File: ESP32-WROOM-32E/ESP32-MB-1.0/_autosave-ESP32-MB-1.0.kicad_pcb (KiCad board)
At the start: 2 copper layers, 125.6 x 91.4 mm, 52 parts, among them J1 Conn_01x19, J10 Conn_01x03_Pin, J11 Conn_01x03_Pin, J12 Conn_01x03_Pin, J13 Conn_01x03_Pin, J14 Conn_01x03_Pin, J15 Conn_01x03_Pin, J16 XT60-M, J2 Conn_01x19, J21 Conn_01x02_Pin, J22 XT60-M, J23 Conn_01x02_Pin, J24 Conn_01x02_Pin, J25 Conn_01x02_Pin, J26 Conn_01x02_Pin, J27 Conn_01x02_Pin, J28 Conn_01x02_Pin, J29 Conn_01x02_Pin, J3 Conn_01x19, J30 XT60-M, J31 Conn_01x02_Pin, J32 Conn_01x02_Pin, J33 Conn_01x11_Pin, J34 Conn_01x02_Pin, J35 Conn_01x02_Pin, J36 Conn_01x02_Pin, J37 Conn_01x02_Pin, J38 Conn_01x02_Pin, J39 Conn_01x02_Pin, J4 Conn_01x11_Pin, J5 Conn_01x11_Pin, J6 XT60-M, J7 Conn_01x19, J8 Conn_01x03_Pin, J9 Conn_01x03_Pin, U1 IRLB3813PBF, U2 IRLB3813PBF, U3 IRLB3813PBF, U4 IRLB3813PBF, U5 IRLB3813PBF, U6 IRLB3813PBF, U7 IRLB3813PBF, U8 IRLB3813PBF, U9 MCP2562-E-P

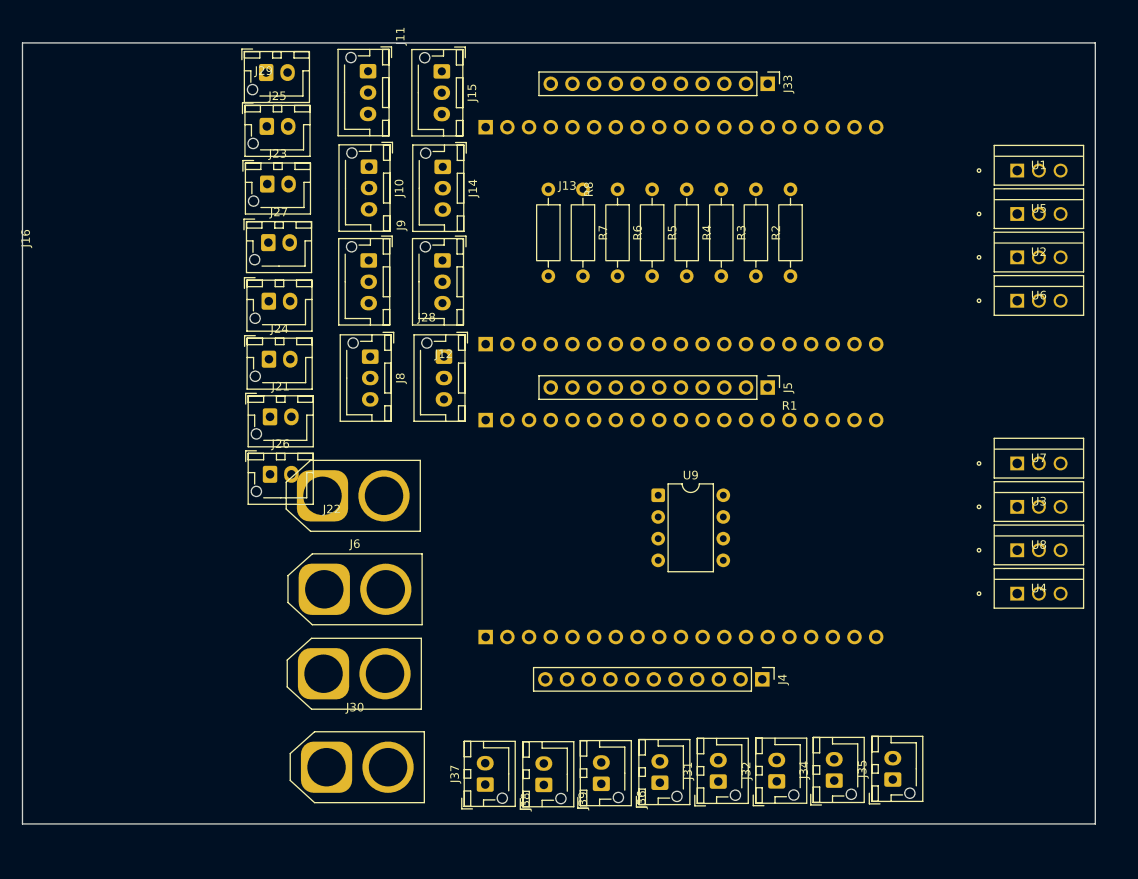
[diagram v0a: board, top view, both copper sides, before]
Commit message: ESP割り当て
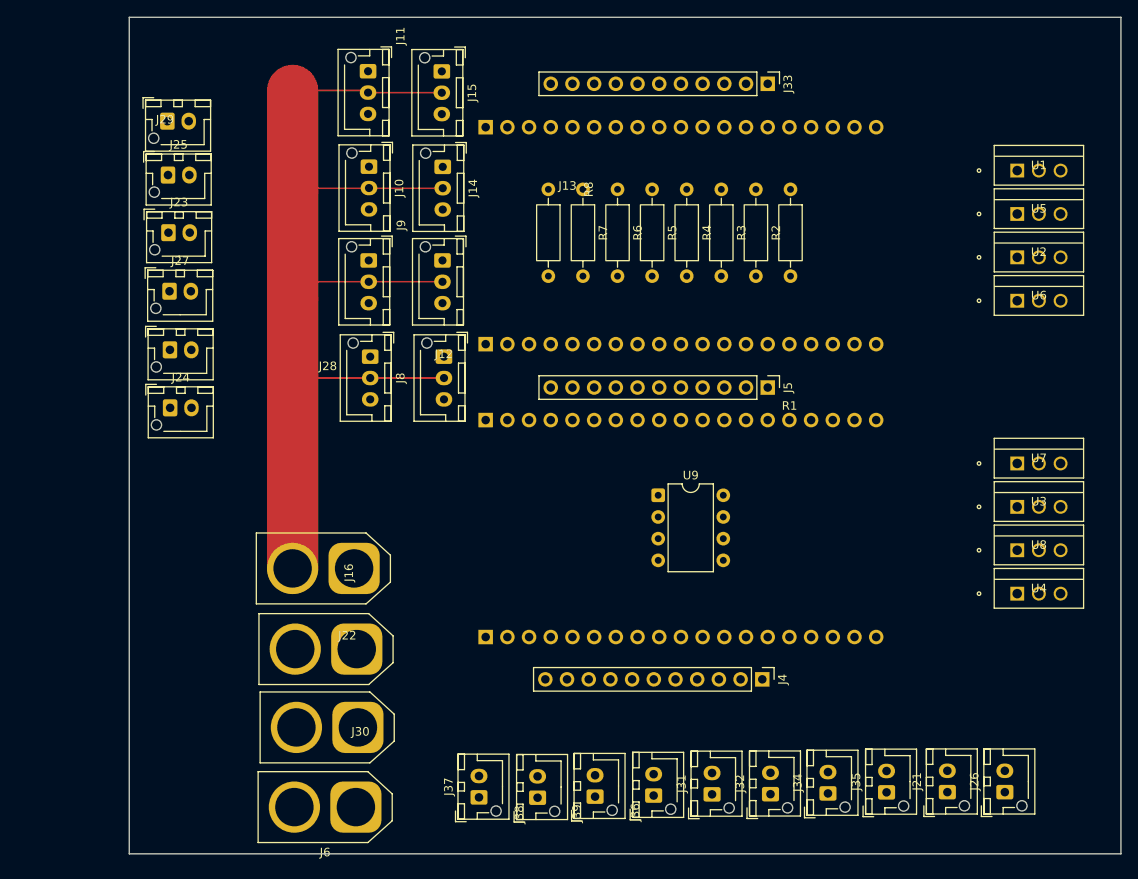
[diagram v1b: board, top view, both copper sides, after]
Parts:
- moved J26 93.7 mm to (234.0, 125.9), turned to 90 degrees
- moved J21 90.7 mm to (227.3, 125.9), turned to 90 degrees
- moved J6 25.8 mm to (158.0, 127.6), turned to 180 degrees
- moved J22 18.4 mm to (158.1, 109.1), turned to 180 degrees
- moved J28 12.9 mm to (136.3, 74.1)
- moved J23 12.9 mm to (136.1, 60.4)
- moved J25 12.9 mm to (136.0, 53.6)
- moved J29 12.9 mm to (136.0, 47.3)
- moved J24 12.9 mm to (136.3, 80.9)
- moved J27 12.9 mm to (136.2, 67.2)
- moved J16 12.8 mm to (157.8, 99.7), turned to 180 degrees
- moved J30 5.93 mm to (158.3, 118.3), turned to 180 degrees
- moved J31 1.67 mm to (199.7, 126.1)
- moved J32 1.67 mm to (206.6, 126.1)
- moved J34 1.67 mm to (213.3, 126.0)
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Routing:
- net +_servo: track 0.00 -> 128.4 mm
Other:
- board size 125.6 x 91.4 mm -> 116.1 x 97.9 mm
